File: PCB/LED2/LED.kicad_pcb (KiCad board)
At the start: 2 copper layers, 70 x 70 mm, 35 parts, among them J1 Conn_01x03, J2 USB-C, U1 ESP32-PICO-MINI-02, U2 QR, U3 MD8942, U4 Barcode, U5 CH340X

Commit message: V Cuts
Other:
- board text added: "2 Designs, 0.8mm, Black"
- board text removed: "2 Designs, 0.8mm, Black, V-Cuts"

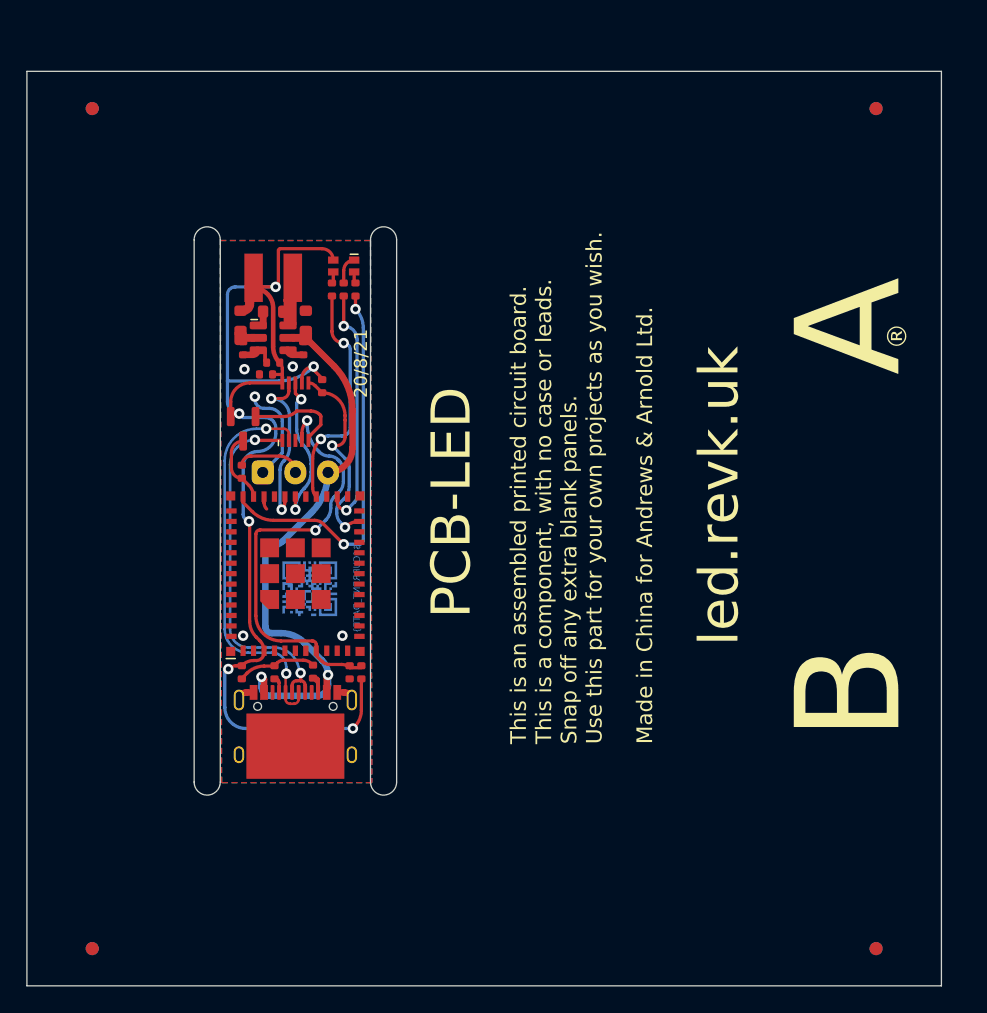
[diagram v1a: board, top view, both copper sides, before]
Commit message: Better Rails
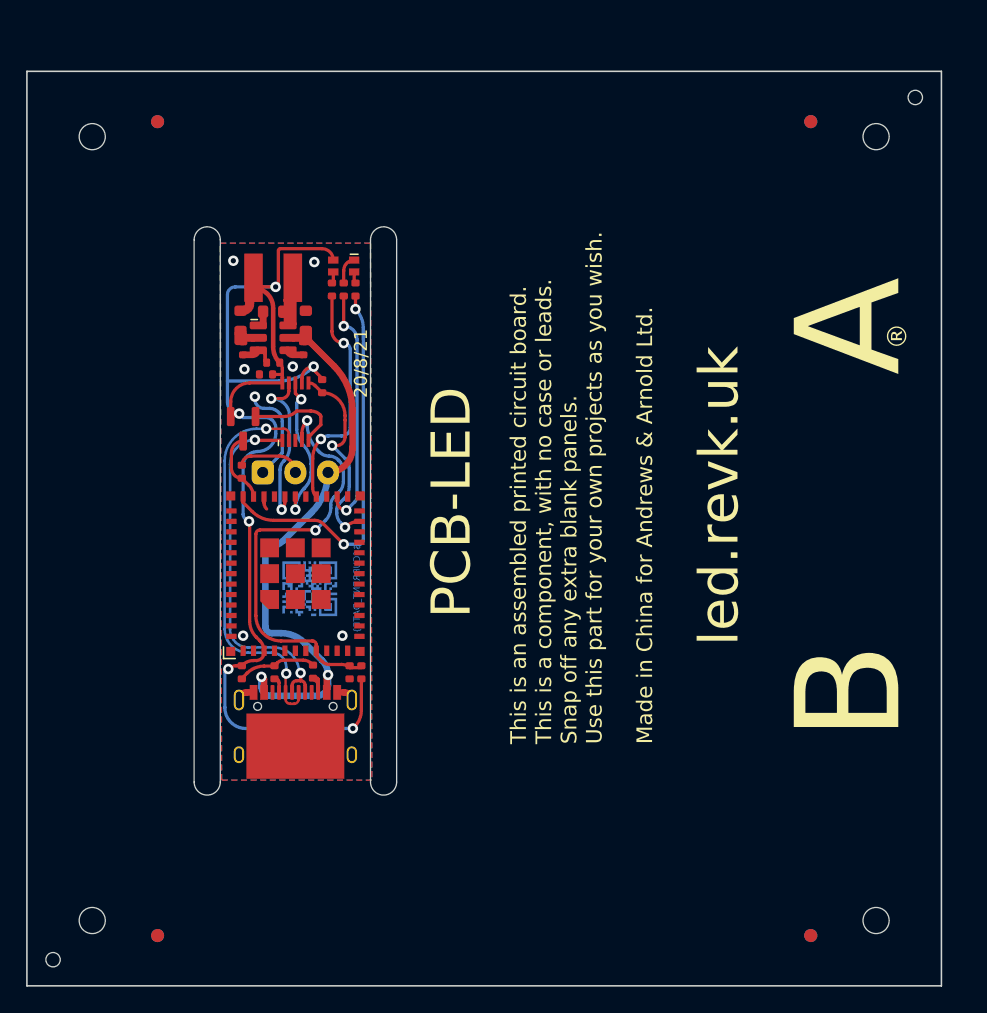
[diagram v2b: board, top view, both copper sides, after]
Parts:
- removed FID1, FID2, FID3, FID4, FID5, FID6, FID7, FID8: Fiducial, Fiducial:Fiducial_1mm_Mask2mm
- added PCB1: 70x70, RevK:PCB7070, F.Cu at (135.0, 65.0)
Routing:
- net GND: vias 5 -> 7
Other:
- outline, holes or cut-outs redrawn
